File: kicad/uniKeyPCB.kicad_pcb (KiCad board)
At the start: 2 copper layers, 84 x 84 mm, 136 parts, among them J1 Conn_01x03_Socket, J10 Conn_01x02_Socket, J2 Conn_01x03_Socket, J3 Conn_01x02_Socket, J4 Conn_01x02_Socket, J5 Conn_01x03_Socket, J6 Conn_01x03_Socket, J9 Conn_01x02_Socket, SW1 SW_CHOC_HS, SW2 SW_MX_HS

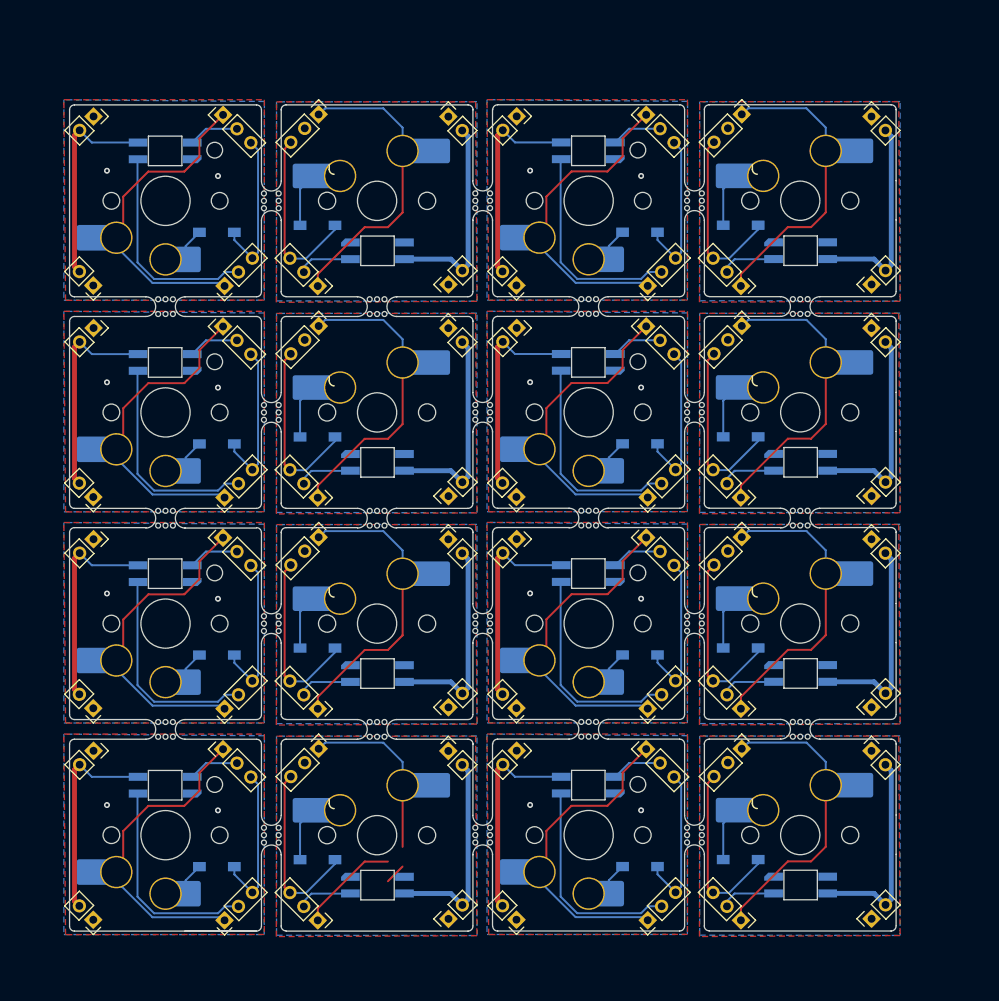
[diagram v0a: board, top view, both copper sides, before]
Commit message: wip
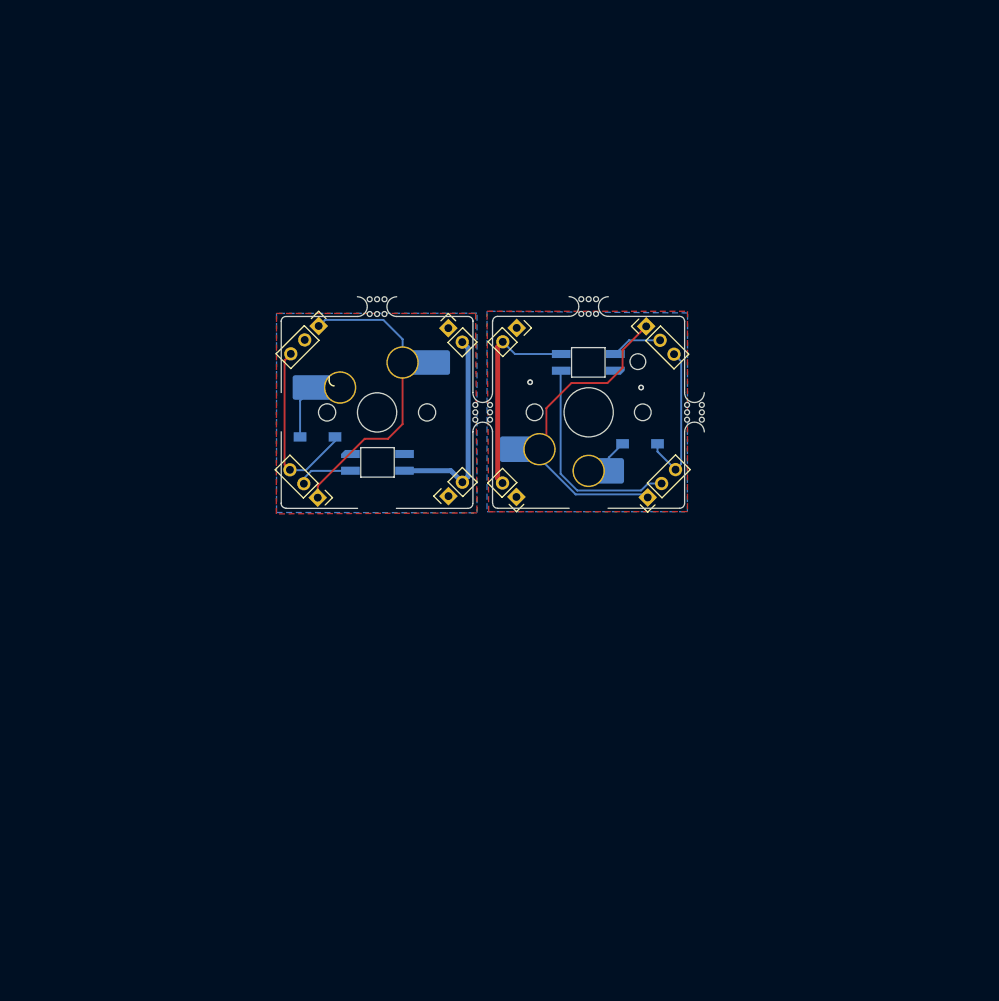
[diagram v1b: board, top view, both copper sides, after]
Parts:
- removed the D1 at (75.5, 130.6)
- removed the D1 at (118.6, 130.6)
- removed the D1 at (75.5, 87.6)
- removed the D1 at (75.5, 109.1)
- removed the D1 at (118.6, 66.1)
- removed the D1 at (75.5, 66.1)
- removed the D1 at (118.6, 109.0)
- removed the D2 at (85.8, 65.4)
- removed the D2 at (128.8, 129.8)
- removed the D2 at (128.8, 65.4)
- removed the D2 at (85.8, 129.8)
- removed the D2 at (128.8, 108.3)
- removed the D2 at (128.8, 86.9)
- removed the D2 at (85.8, 108.3)
- removed the J1 at (119.2, 54.2)
- removed the J1 at (119.2, 118.6)
- removed the J1 at (76.2, 54.2)
- removed the J1 at (76.2, 75.7)
- removed the J1 at (119.2, 97.1)
- removed the J1 at (76.2, 97.1)
- removed the J1 at (76.2, 118.6)
- removed the J10 at (63.0, 136.0)
- removed the J10 at (106.0, 114.5)
- removed the J10 at (106.0, 71.5)
- removed the J10 at (63.0, 93.0)
- removed the J10 at (63.0, 114.5)
- removed the J10 at (106.0, 135.9)
- removed the J10 at (63.0, 71.5)
- removed the J2 at (76.3, 71.5)
- removed the J2 at (76.3, 114.5)
- removed the J2 at (119.3, 136.0)
- removed the J2 at (76.3, 136.0)
- removed the J2 at (119.3, 71.5)
- removed the J2 at (76.3, 93.0)
- removed the J2 at (119.3, 114.5)
- removed the J3 at (142.1, 71.4)
- removed the J3 at (99.1, 114.4)
- removed the J3 at (142.1, 135.9)
- removed the J3 at (99.1, 135.9)
- removed the J3 at (142.1, 114.4)
- removed the J3 at (99.1, 71.4)
- removed the J3 at (142.1, 92.9)
- removed the J4 at (142.1, 97.3)
- removed the J4 at (142.1, 118.8)
- removed the J4 at (99.1, 54.3)
- removed the J4 at (142.1, 75.8)
- removed the J4 at (99.1, 118.8)
- removed the J4 at (142.1, 54.3)
- removed the J4 at (99.1, 97.3)
- removed the J5 at (128.8, 114.5)
- removed the J5 at (85.8, 71.6)
- removed the J5 at (85.8, 136.0)
- removed the J5 at (85.8, 114.5)
- removed the J5 at (128.8, 136.0)
- removed the J5 at (128.8, 93.0)
- removed the J5 at (128.8, 71.5)
- removed the J6 at (85.9, 118.6)
- removed the J6 at (85.9, 54.1)
- removed the J6 at (128.9, 54.1)
- removed the J6 at (128.9, 118.6)
- removed the J6 at (128.9, 75.6)
- removed the J6 at (128.9, 97.1)
- removed the J6 at (85.9, 97.1)
- removed the J9 at (63.0, 118.8)
- removed the J9 at (106.0, 97.3)
- removed the J9 at (106.0, 54.3)
- removed the J9 at (63.0, 97.3)
- removed the J9 at (63.0, 75.8)
- removed the J9 at (106.0, 118.8)
- removed the J9 at (63.0, 54.3)
- removed the LED1 at (113.3, 122.3)
- removed the LED1 at (70.3, 100.8)
- removed the LED1 at (113.3, 57.8)
- removed the LED1 at (70.3, 79.3)
- removed the LED1 at (113.3, 100.8)
- removed the LED1 at (70.3, 57.8)
- removed the LED1 at (70.3, 122.3)
- removed the LED2 at (134.8, 89.5)
- removed the LED2 at (134.8, 110.9)
- removed the LED2 at (91.8, 110.9)
- removed the LED2 at (91.8, 132.4)
- removed the LED2 at (91.8, 68.0)
- removed the LED2 at (134.8, 68.0)
- removed the LED2 at (134.8, 132.4)
- removed the SW1 at (70.3, 62.9)
- removed the SW1 at (113.3, 127.3)
- removed the SW1 at (113.3, 105.8)
- removed the SW1 at (70.3, 105.9)
- removed the SW1 at (113.3, 62.9)
- removed the SW1 at (70.3, 127.4)
- removed the SW1 at (70.3, 84.4)
- removed the SW2 at (91.8, 62.9)
- removed the SW2 at (134.8, 127.3)
- removed the SW2 at (134.8, 105.8)
- removed the SW2 at (134.8, 62.9)
- removed the SW2 at (91.8, 127.4)
- removed the SW2 at (134.8, 84.4)
- removed the SW2 at (91.8, 105.9)
- removed the mouse-bite-2mm-slot at (113.3, 95.1)
- removed the mouse-bite-2mm-slot at (81.1, 62.9)
- removed the mouse-bite-2mm-slot at (91.8, 95.2)
- removed the mouse-bite-2mm-slot at (70.3, 95.2)
- removed the mouse-bite-2mm-slot at (102.6, 62.9)
- removed the mouse-bite-2mm-slot at (102.6, 127.3)
- removed the mouse-bite-2mm-slot at (102.6, 105.8)
- removed the mouse-bite-2mm-slot at (70.3, 73.7)
- removed the mouse-bite-2mm-slot at (124.1, 127.3)
- removed the mouse-bite-2mm-slot at (124.1, 105.8)
- removed the mouse-bite-2mm-slot at (91.8, 116.6)
- removed the mouse-bite-2mm-slot at (134.8, 73.6)
- removed the mouse-bite-2mm-slot at (113.3, 116.6)
- removed the mouse-bite-2mm-slot at (81.1, 127.4)
- removed the mouse-bite-2mm-slot at (81.1, 84.4)
- removed the mouse-bite-2mm-slot at (134.8, 116.6)
- removed the mouse-bite-2mm-slot at (134.8, 95.1)
- removed the mouse-bite-2mm-slot at (124.1, 62.9)
- removed the mouse-bite-2mm-slot at (81.1, 105.9)
- removed the mouse-bite-2mm-slot at (70.3, 116.6)
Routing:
- net VCC: track 338.8 -> 42.3 mm
- net col0: track 262.1 -> 32.8 mm
- net col1: track 243.6 -> 30.7 mm
- net LED0_out: track 174.1 -> 21.8 mm
- net row1: track 148.0 -> 18.5 mm
- net row0: track 125.2 -> 15.6 mm
- net LED1_in: track 45.0 -> 5.63 mm
- net Net-(D2-A): track 44.6 -> 5.58 mm
- net LED0_in: track 41.0 -> 5.13 mm
- net Net-(D1-A): track 26.6 -> 3.33 mm
- net GND: track 2.11 -> 0.00 mm, vias 16 -> 2
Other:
- board size 84 x 84 mm -> 41 x 19.5 mm
- board text removed: "in"

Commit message: fixed a bug
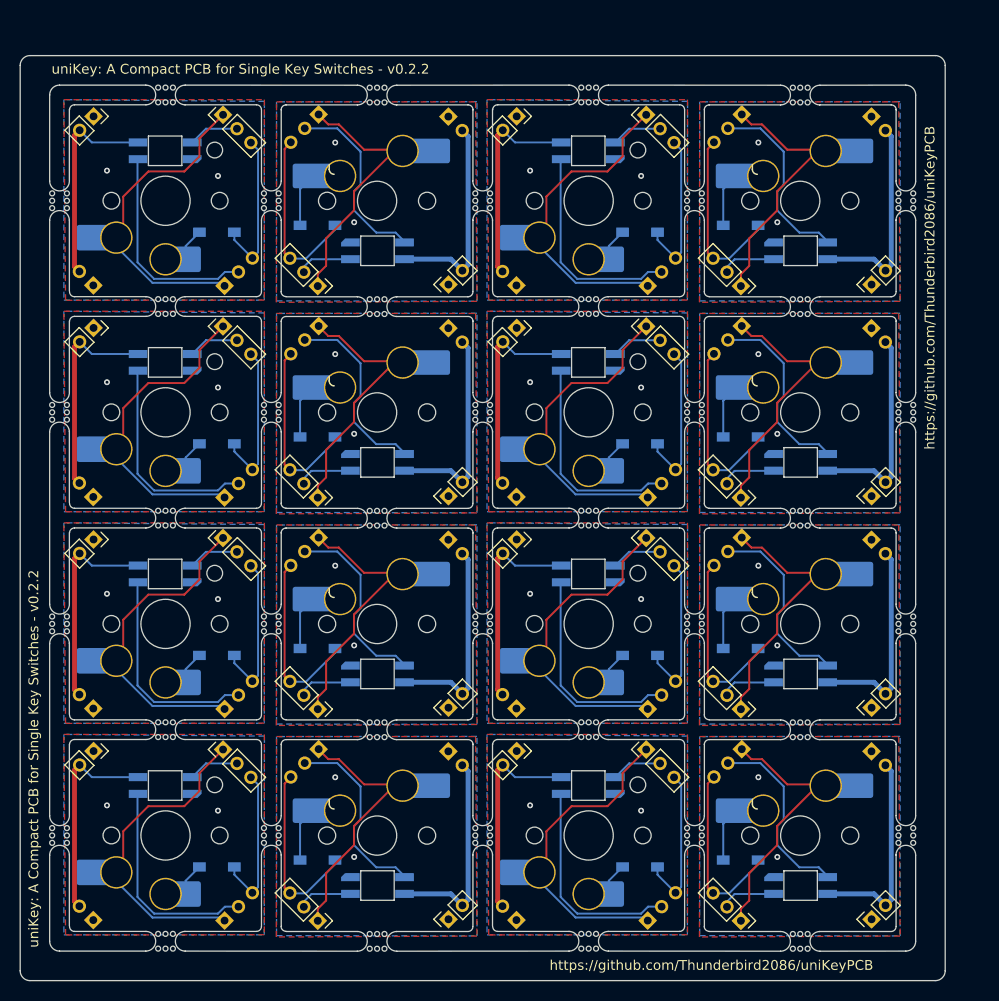
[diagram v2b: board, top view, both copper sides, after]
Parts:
- added D1: 1N4148WS, TB2086_SMD:D3_SMD, F.Cu at (75.6, 66.1)
- added D1: 1N4148WS, TB2086_SMD:D3_SMD, F.Cu at (118.6, 66.1)
- added D1: 1N4148WS, TB2086_SMD:D3_SMD, F.Cu at (75.6, 109.1)
- added D1: 1N4148WS, TB2086_SMD:D3_SMD, F.Cu at (75.6, 87.6)
- added D1: 1N4148WS, TB2086_SMD:D3_SMD, F.Cu at (75.6, 130.6)
- added D1: 1N4148WS, TB2086_SMD:D3_SMD, F.Cu at (118.6, 109.1)
- added D1: 1N4148WS, TB2086_SMD:D3_SMD, F.Cu at (118.6, 130.6)
- added D2: 1N4148WS, TB2086_SMD:D3_SMD, F.Cu at (85.8, 65.4)
- added D2: 1N4148WS, TB2086_SMD:D3_SMD, F.Cu at (85.8, 108.4)
- added D2: 1N4148WS, TB2086_SMD:D3_SMD, F.Cu at (128.8, 65.4)
- added D2: 1N4148WS, TB2086_SMD:D3_SMD, F.Cu at (128.8, 86.9)
- added D2: 1N4148WS, TB2086_SMD:D3_SMD, F.Cu at (128.8, 108.4)
- added D2: 1N4148WS, TB2086_SMD:D3_SMD, F.Cu at (85.8, 129.9)
- added D2: 1N4148WS, TB2086_SMD:D3_SMD, F.Cu at (128.8, 129.9)
- added J1: Conn_01x03_Socket, Connector_PinHeader_2.00mm:PinHeader_1x03_P2.00mm_Vertical, F.Cu at (119.2, 54.2)
- added J1: Conn_01x03_Socket, Connector_PinHeader_2.00mm:PinHeader_1x03_P2.00mm_Vertical, F.Cu at (119.2, 118.7)
- added J1: Conn_01x03_Socket, Connector_PinHeader_2.00mm:PinHeader_1x03_P2.00mm_Vertical, F.Cu at (119.2, 97.2)
- added J1: Conn_01x03_Socket, Connector_PinHeader_2.00mm:PinHeader_1x03_P2.00mm_Vertical, F.Cu at (76.2, 54.2)
- added J1: Conn_01x03_Socket, Connector_PinHeader_2.00mm:PinHeader_1x03_P2.00mm_Vertical, F.Cu at (76.2, 118.7)
- added J1: Conn_01x03_Socket, Connector_PinHeader_2.00mm:PinHeader_1x03_P2.00mm_Vertical, F.Cu at (76.2, 75.7)
- added J1: Conn_01x03_Socket, Connector_PinHeader_2.00mm:PinHeader_1x03_P2.00mm_Vertical, F.Cu at (76.2, 97.2)
- added J10: Conn_01x02_Socket, Connector_PinSocket_2.00mm:PinSocket_1x02_P2.00mm_Vertical, B.Cu at (106.0, 114.5)
- added J10: Conn_01x02_Socket, Connector_PinSocket_2.00mm:PinSocket_1x02_P2.00mm_Vertical, B.Cu at (63.0, 93.0)
- added J10: Conn_01x02_Socket, Connector_PinSocket_2.00mm:PinSocket_1x02_P2.00mm_Vertical, B.Cu at (63.0, 136.0)
- added J10: Conn_01x02_Socket, Connector_PinSocket_2.00mm:PinSocket_1x02_P2.00mm_Vertical, B.Cu at (106.0, 136.0)
- added J10: Conn_01x02_Socket, Connector_PinSocket_2.00mm:PinSocket_1x02_P2.00mm_Vertical, B.Cu at (63.0, 71.5)
- added J10: Conn_01x02_Socket, Connector_PinSocket_2.00mm:PinSocket_1x02_P2.00mm_Vertical, B.Cu at (106.0, 71.5)
- added J10: Conn_01x02_Socket, Connector_PinSocket_2.00mm:PinSocket_1x02_P2.00mm_Vertical, B.Cu at (63.0, 114.5)
- added J2: Conn_01x03_Socket, Connector_PinHeader_2.00mm:PinHeader_1x03_P2.00mm_Vertical, B.Cu at (119.3, 71.5)
- added J2: Conn_01x03_Socket, Connector_PinHeader_2.00mm:PinHeader_1x03_P2.00mm_Vertical, B.Cu at (76.3, 136.0)
- added J2: Conn_01x03_Socket, Connector_PinHeader_2.00mm:PinHeader_1x03_P2.00mm_Vertical, B.Cu at (119.3, 114.5)
- added J2: Conn_01x03_Socket, Connector_PinHeader_2.00mm:PinHeader_1x03_P2.00mm_Vertical, B.Cu at (119.3, 136.0)
- added J2: Conn_01x03_Socket, Connector_PinHeader_2.00mm:PinHeader_1x03_P2.00mm_Vertical, B.Cu at (76.3, 114.5)
- added J2: Conn_01x03_Socket, Connector_PinHeader_2.00mm:PinHeader_1x03_P2.00mm_Vertical, B.Cu at (76.3, 93.0)
- added J2: Conn_01x03_Socket, Connector_PinHeader_2.00mm:PinHeader_1x03_P2.00mm_Vertical, B.Cu at (76.3, 71.5)
- added J3: Conn_01x02_Socket, Connector_PinSocket_2.00mm:PinSocket_1x02_P2.00mm_Vertical, F.Cu at (142.1, 92.9)
- added J3: Conn_01x02_Socket, Connector_PinSocket_2.00mm:PinSocket_1x02_P2.00mm_Vertical, F.Cu at (99.1, 135.9)
- added J3: Conn_01x02_Socket, Connector_PinSocket_2.00mm:PinSocket_1x02_P2.00mm_Vertical, F.Cu at (99.1, 71.4)
- added J3: Conn_01x02_Socket, Connector_PinSocket_2.00mm:PinSocket_1x02_P2.00mm_Vertical, F.Cu at (99.1, 114.4)
- added J3: Conn_01x02_Socket, Connector_PinSocket_2.00mm:PinSocket_1x02_P2.00mm_Vertical, F.Cu at (142.1, 114.4)
- added J3: Conn_01x02_Socket, Connector_PinSocket_2.00mm:PinSocket_1x02_P2.00mm_Vertical, F.Cu at (142.1, 71.4)
- added J3: Conn_01x02_Socket, Connector_PinSocket_2.00mm:PinSocket_1x02_P2.00mm_Vertical, F.Cu at (142.1, 135.9)
- added J4: Conn_01x02_Socket, Connector_PinSocket_2.00mm:PinSocket_1x02_P2.00mm_Vertical, B.Cu at (99.1, 97.3)
- added J4: Conn_01x02_Socket, Connector_PinSocket_2.00mm:PinSocket_1x02_P2.00mm_Vertical, B.Cu at (142.1, 75.8)
- added J4: Conn_01x02_Socket, Connector_PinSocket_2.00mm:PinSocket_1x02_P2.00mm_Vertical, B.Cu at (142.1, 97.3)
- added J4: Conn_01x02_Socket, Connector_PinSocket_2.00mm:PinSocket_1x02_P2.00mm_Vertical, B.Cu at (99.1, 118.8)
- added J4: Conn_01x02_Socket, Connector_PinSocket_2.00mm:PinSocket_1x02_P2.00mm_Vertical, B.Cu at (142.1, 54.3)
- added J4: Conn_01x02_Socket, Connector_PinSocket_2.00mm:PinSocket_1x02_P2.00mm_Vertical, B.Cu at (99.1, 54.3)
- added J4: Conn_01x02_Socket, Connector_PinSocket_2.00mm:PinSocket_1x02_P2.00mm_Vertical, B.Cu at (142.1, 118.8)
- added J5: Conn_01x03_Socket, Connector_PinHeader_2.00mm:PinHeader_1x03_P2.00mm_Vertical, F.Cu at (128.8, 114.6)
- added J5: Conn_01x03_Socket, Connector_PinHeader_2.00mm:PinHeader_1x03_P2.00mm_Vertical, F.Cu at (85.8, 71.6)
- added J5: Conn_01x03_Socket, Connector_PinHeader_2.00mm:PinHeader_1x03_P2.00mm_Vertical, F.Cu at (128.8, 136.1)
- added J5: Conn_01x03_Socket, Connector_PinHeader_2.00mm:PinHeader_1x03_P2.00mm_Vertical, F.Cu at (85.8, 114.6)
- added J5: Conn_01x03_Socket, Connector_PinHeader_2.00mm:PinHeader_1x03_P2.00mm_Vertical, F.Cu at (128.8, 93.1)
- added J5: Conn_01x03_Socket, Connector_PinHeader_2.00mm:PinHeader_1x03_P2.00mm_Vertical, F.Cu at (128.8, 71.6)
- added J5: Conn_01x03_Socket, Connector_PinHeader_2.00mm:PinHeader_1x03_P2.00mm_Vertical, F.Cu at (85.8, 136.1)
- added J6: Conn_01x03_Socket, Connector_PinHeader_2.00mm:PinHeader_1x03_P2.00mm_Vertical, B.Cu at (128.9, 97.1)
- added J6: Conn_01x03_Socket, Connector_PinHeader_2.00mm:PinHeader_1x03_P2.00mm_Vertical, B.Cu at (85.9, 54.1)
- added J6: Conn_01x03_Socket, Connector_PinHeader_2.00mm:PinHeader_1x03_P2.00mm_Vertical, B.Cu at (128.9, 75.6)
- added J6: Conn_01x03_Socket, Connector_PinHeader_2.00mm:PinHeader_1x03_P2.00mm_Vertical, B.Cu at (128.9, 54.1)
- added J6: Conn_01x03_Socket, Connector_PinHeader_2.00mm:PinHeader_1x03_P2.00mm_Vertical, B.Cu at (128.9, 118.6)
- added J6: Conn_01x03_Socket, Connector_PinHeader_2.00mm:PinHeader_1x03_P2.00mm_Vertical, B.Cu at (85.9, 118.6)
- added J6: Conn_01x03_Socket, Connector_PinHeader_2.00mm:PinHeader_1x03_P2.00mm_Vertical, B.Cu at (85.9, 97.1)
- added J9: Conn_01x02_Socket, Connector_PinSocket_2.00mm:PinSocket_1x02_P2.00mm_Vertical, F.Cu at (63.0, 75.8)
- added J9: Conn_01x02_Socket, Connector_PinSocket_2.00mm:PinSocket_1x02_P2.00mm_Vertical, F.Cu at (106.0, 54.3)
- added J9: Conn_01x02_Socket, Connector_PinSocket_2.00mm:PinSocket_1x02_P2.00mm_Vertical, F.Cu at (63.0, 97.3)
- added J9: Conn_01x02_Socket, Connector_PinSocket_2.00mm:PinSocket_1x02_P2.00mm_Vertical, F.Cu at (106.0, 118.8)
- added J9: Conn_01x02_Socket, Connector_PinSocket_2.00mm:PinSocket_1x02_P2.00mm_Vertical, F.Cu at (106.0, 97.3)
- added J9: Conn_01x02_Socket, Connector_PinSocket_2.00mm:PinSocket_1x02_P2.00mm_Vertical, F.Cu at (63.0, 118.8)
- added J9: Conn_01x02_Socket, Connector_PinSocket_2.00mm:PinSocket_1x02_P2.00mm_Vertical, F.Cu at (63.0, 54.3)
- added LED1: SK6812MINI-E, TB2086_LED:LED_SW_SK6812-E-rot, F.Cu at (113.3, 100.8)
- added LED1: SK6812MINI-E, TB2086_LED:LED_SW_SK6812-E-rot, F.Cu at (70.3, 100.8)
- added LED1: SK6812MINI-E, TB2086_LED:LED_SW_SK6812-E-rot, F.Cu at (70.3, 79.3)
- added LED1: SK6812MINI-E, TB2086_LED:LED_SW_SK6812-E-rot, F.Cu at (113.3, 57.8)
- added LED1: SK6812MINI-E, TB2086_LED:LED_SW_SK6812-E-rot, F.Cu at (113.3, 122.3)
- added LED1: SK6812MINI-E, TB2086_LED:LED_SW_SK6812-E-rot, F.Cu at (70.3, 122.3)
- added LED1: SK6812MINI-E, TB2086_LED:LED_SW_SK6812-E-rot, F.Cu at (70.3, 57.8)
- added LED2: SK6812MINI-E, TB2086_LED:LED_SW_SK6812-E-rot, F.Cu at (134.8, 89.5)
- added LED2: SK6812MINI-E, TB2086_LED:LED_SW_SK6812-E-rot, F.Cu at (134.8, 68.0)
- added LED2: SK6812MINI-E, TB2086_LED:LED_SW_SK6812-E-rot, F.Cu at (134.8, 111.0)
- added LED2: SK6812MINI-E, TB2086_LED:LED_SW_SK6812-E-rot, F.Cu at (134.8, 132.5)
- added LED2: SK6812MINI-E, TB2086_LED:LED_SW_SK6812-E-rot, F.Cu at (91.8, 68.0)
- added LED2: SK6812MINI-E, TB2086_LED:LED_SW_SK6812-E-rot, F.Cu at (91.8, 111.0)
- added LED2: SK6812MINI-E, TB2086_LED:LED_SW_SK6812-E-rot, F.Cu at (91.8, 132.5)
- added SW1: SW_CHOC_HS, TB2086_KEYSWITCH:SW_choc_v1_v2_HS_1u, F.Cu at (113.3, 105.9)
- added SW1: SW_CHOC_HS, TB2086_KEYSWITCH:SW_choc_v1_v2_HS_1u, F.Cu at (70.3, 84.4)
- added SW1: SW_CHOC_HS, TB2086_KEYSWITCH:SW_choc_v1_v2_HS_1u, F.Cu at (70.3, 62.9)
- added SW1: SW_CHOC_HS, TB2086_KEYSWITCH:SW_choc_v1_v2_HS_1u, F.Cu at (70.3, 105.9)
- added SW1: SW_CHOC_HS, TB2086_KEYSWITCH:SW_choc_v1_v2_HS_1u, F.Cu at (70.3, 127.4)
- added SW1: SW_CHOC_HS, TB2086_KEYSWITCH:SW_choc_v1_v2_HS_1u, F.Cu at (113.3, 127.4)
- added SW1: SW_CHOC_HS, TB2086_KEYSWITCH:SW_choc_v1_v2_HS_1u, F.Cu at (113.3, 62.9)
- added SW2: SW_MX_HS, TB2086_KEYSWITCH:SW_MX_HS_1u, F.Cu at (91.8, 127.4)
- added SW2: SW_MX_HS, TB2086_KEYSWITCH:SW_MX_HS_1u, F.Cu at (134.8, 62.9)
- added SW2: SW_MX_HS, TB2086_KEYSWITCH:SW_MX_HS_1u, F.Cu at (134.8, 105.9)
- added SW2: SW_MX_HS, TB2086_KEYSWITCH:SW_MX_HS_1u, F.Cu at (134.8, 127.4)
- added SW2: SW_MX_HS, TB2086_KEYSWITCH:SW_MX_HS_1u, F.Cu at (134.8, 84.4)
- added SW2: SW_MX_HS, TB2086_KEYSWITCH:SW_MX_HS_1u, F.Cu at (91.8, 105.9)
- added SW2: SW_MX_HS, TB2086_KEYSWITCH:SW_MX_HS_1u, F.Cu at (91.8, 62.9)
- added mouse-bite-2mm-slot: VAL**, Mouse_Bite:mouse-bite-2mm-slot, F.Cu at (81.1, 84.4)
- added mouse-bite-2mm-slot: VAL**, Mouse_Bite:mouse-bite-2mm-slot, F.Cu at (113.3, 116.6)
- added mouse-bite-2mm-slot: VAL**, Mouse_Bite:mouse-bite-2mm-slot, F.Cu at (91.8, 116.7)
- added mouse-bite-2mm-slot: VAL**, Mouse_Bite:mouse-bite-2mm-slot, F.Cu at (102.6, 62.9)
- added mouse-bite-2mm-slot: VAL**, Mouse_Bite:mouse-bite-2mm-slot, F.Cu at (59.6, 127.4)
- added mouse-bite-2mm-slot: VAL**, Mouse_Bite:mouse-bite-2mm-slot, F.Cu at (124.1, 62.9)
- added mouse-bite-2mm-slot: VAL**, Mouse_Bite:mouse-bite-2mm-slot, F.Cu at (102.6, 105.9)
- added mouse-bite-2mm-slot: VAL**, Mouse_Bite:mouse-bite-2mm-slot, F.Cu at (145.6, 84.4)
- added mouse-bite-2mm-slot: VAL**, Mouse_Bite:mouse-bite-2mm-slot, F.Cu at (145.6, 62.9)
- added mouse-bite-2mm-slot: VAL**, Mouse_Bite:mouse-bite-2mm-slot, F.Cu at (124.1, 127.4)
- added mouse-bite-2mm-slot: VAL**, Mouse_Bite:mouse-bite-2mm-slot, F.Cu at (145.6, 127.4)
- added mouse-bite-2mm-slot: VAL**, Mouse_Bite:mouse-bite-2mm-slot, F.Cu at (81.1, 127.4)
- added mouse-bite-2mm-slot: VAL**, Mouse_Bite:mouse-bite-2mm-slot, F.Cu at (113.3, 138.1)
- added mouse-bite-2mm-slot: VAL**, Mouse_Bite:mouse-bite-2mm-slot, F.Cu at (70.3, 73.6)
- added mouse-bite-2mm-slot: VAL**, Mouse_Bite:mouse-bite-2mm-slot, F.Cu at (134.8, 116.7)
- added mouse-bite-2mm-slot: VAL**, Mouse_Bite:mouse-bite-2mm-slot, F.Cu at (81.1, 62.9)
- added mouse-bite-2mm-slot: VAL**, Mouse_Bite:mouse-bite-2mm-slot, F.Cu at (70.3, 52.1)
- added mouse-bite-2mm-slot: VAL**, Mouse_Bite:mouse-bite-2mm-slot, F.Cu at (134.8, 138.2)
- added mouse-bite-2mm-slot: VAL**, Mouse_Bite:mouse-bite-2mm-slot, F.Cu at (113.3, 52.1)
- added mouse-bite-2mm-slot: VAL**, Mouse_Bite:mouse-bite-2mm-slot, F.Cu at (134.8, 73.7)
- added mouse-bite-2mm-slot: VAL**, Mouse_Bite:mouse-bite-2mm-slot, F.Cu at (113.3, 95.1)
- added mouse-bite-2mm-slot: VAL**, Mouse_Bite:mouse-bite-2mm-slot, F.Cu at (70.3, 138.1)
- added mouse-bite-2mm-slot: VAL**, Mouse_Bite:mouse-bite-2mm-slot, F.Cu at (59.6, 105.9)
- added mouse-bite-2mm-slot: VAL**, Mouse_Bite:mouse-bite-2mm-slot, F.Cu at (59.6, 84.4)
- added mouse-bite-2mm-slot: VAL**, Mouse_Bite:mouse-bite-2mm-slot, F.Cu at (91.8, 138.2)
- added mouse-bite-2mm-slot: VAL**, Mouse_Bite:mouse-bite-2mm-slot, F.Cu at (70.3, 116.6)
- added mouse-bite-2mm-slot: VAL**, Mouse_Bite:mouse-bite-2mm-slot, F.Cu at (145.6, 105.9)
- added mouse-bite-2mm-slot: VAL**, Mouse_Bite:mouse-bite-2mm-slot, F.Cu at (59.6, 62.9)
- added mouse-bite-2mm-slot: VAL**, Mouse_Bite:mouse-bite-2mm-slot, F.Cu at (91.8, 95.2)
- added mouse-bite-2mm-slot: VAL**, Mouse_Bite:mouse-bite-2mm-slot, F.Cu at (134.8, 95.2)
- added mouse-bite-2mm-slot: VAL**, Mouse_Bite:mouse-bite-2mm-slot, F.Cu at (134.8, 52.1)
- added mouse-bite-2mm-slot: VAL**, Mouse_Bite:mouse-bite-2mm-slot, F.Cu at (124.1, 105.9)
- added mouse-bite-2mm-slot: VAL**, Mouse_Bite:mouse-bite-2mm-slot, F.Cu at (102.6, 127.4)
- added mouse-bite-2mm-slot: VAL**, Mouse_Bite:mouse-bite-2mm-slot, F.Cu at (70.3, 95.1)
- added mouse-bite-2mm-slot: VAL**, Mouse_Bite:mouse-bite-2mm-slot, F.Cu at (81.1, 105.9)
- added mouse-bite-2mm-slot: VAL**, Mouse_Bite:mouse-bite-2mm-slot, F.Cu at (91.8, 52.1)
- J10, J2, J4, J6: moved to B.Cu
- turned J10 to 45 degrees
- turned J2 to -45 degrees
- turned J4 to -135 degrees
- turned J6 to 135 degrees
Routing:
- net VCC: track 42.3 -> 338.8 mm
- net col0: track 32.8 -> 262.1 mm
- net col1: track 30.7 -> 223.0 mm
- net LED1_out: track 0.00 -> 155.5 mm
- net LED0_out: track 21.8 -> 174.1 mm
- net row1: track 18.5 -> 148.0 mm
- net row0: track 15.6 -> 125.2 mm
- net LED1_in: track 5.63 -> 45.0 mm
- net Net-(D2-A): track 5.58 -> 44.6 mm
- net LED0_in: track 5.13 -> 41.0 mm
- net Net-(D1-A): track 3.33 -> 26.6 mm
- net GND: vias 2 -> 32
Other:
- board size 41 x 19.5 mm -> 94 x 94 mm
- board text added: "<- VCC ->"
- board text added: "<- row ->"
- board text added: "Whether you're a experienced keyboard builder or a beginner, uniKey provides a convenient solution for creating"
- board text added: "https://github.com/Thunderbird2086/uniKeyPCB"
- board text added: "in"
- board text added: "uniKey: A Compact PCB for Single Key Switches - v0.2.2"
- board text added: "unique and personalized keyboards. Happy building!"
- board text added: "v0.2.2"
- board text removed: "led in"
- board text removed: "row"
